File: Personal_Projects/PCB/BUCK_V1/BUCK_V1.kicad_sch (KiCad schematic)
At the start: 10 parts, among them J1 Conn_01x03_Socket, U1 AP62150WU

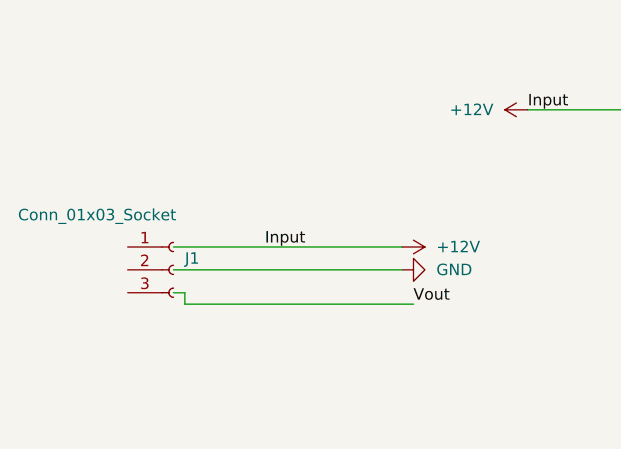
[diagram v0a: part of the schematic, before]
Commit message: lab7
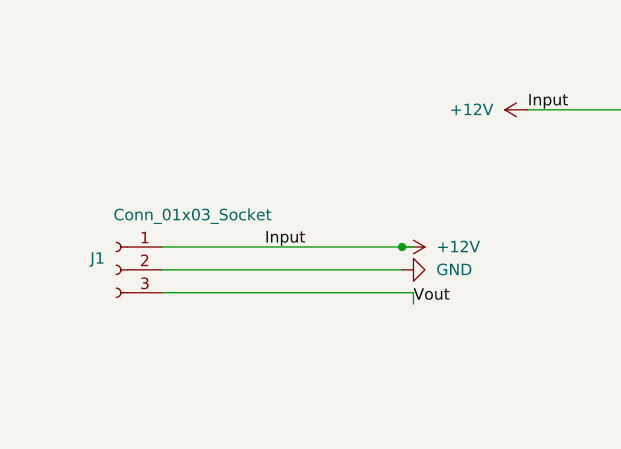
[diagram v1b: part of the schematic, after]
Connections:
- net +12V: now also J1.1 (Pin_1)
- net GND: now also J1.2 (Pin_2)
- net Vout: now also J1.3 (Pin_3)
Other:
- moved on the sheet: J1
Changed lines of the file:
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@@
+	)
+	(junction
+		(at 57.15 60.96)
+		(diameter 0)
+		(color 0 0 0 0)
 	)
 	(junction
@@
 	(wire
 		(pts
-			(xy 31.75 63.5) (xy 57.15 63.5)
+			(xy 30.48 66.04) (xy 58.42 66.04)
 		)
 		(stroke
@@
 	(wire
 		(pts
-			(xy 31.75 66.04) (xy 33.02 66.04)
-		)
-		(stroke
-			(width 0)
-			(type default)
-		)
-	)
-	(wire
-		(pts
 			(xy 146.05 41.91) (xy 166.37 41.91)
 		)
@@
 	(wire
 		(pts
-			(xy 31.75 60.96) (xy 57.15 60.96)
-		)
-		(stroke
-			(width 0)
-			(type default)
-		)
-	)
-	(wire
-		(pts
 			(xy 111.76 72.39) (xy 111.76 74.93)
 		)
@@
 	(wire
 		(pts
+			(xy 57.15 60.96) (xy 58.42 60.96)
+		)
+		(stroke
+			(width 0)
+			(type default)
+		)
+	)
+	(wire
+		(pts
 			(xy 121.92 45.72) (xy 121.92 41.91)
 		)
@@
 	(wire
 		(pts
+			(xy 30.48 60.96) (xy 57.15 60.96)
+		)
+		(stroke
+			(width 0)
+			(type default)
+		)
+	)
+	(wire
+		(pts
 			(xy 166.37 54.61) (xy 166.37 72.39)
 		)
@@
 	(wire
 		(pts
-			(xy 33.02 66.04) (xy 33.02 67.31)
-		)
-		(stroke
-			(width 0)
-			(type default)
-		)
-	)
-	(wire
-		(pts
-			(xy 33.02 67.31) (xy 58.42 67.31)
+			(xy 58.42 66.04) (xy 58.42 67.31)
 		)
 		(stroke
@@
 		(pts
 			(xy 166.37 41.91) (xy 166.37 49.53)
+		)
+		(stroke
+			(width 0)
+			(type default)
+		)
+	)
+	(wire
+		(pts
+			(xy 30.48 63.5) (xy 57.15 63.5)
 		)
 		(stroke
@@
 	(symbol
 		(lib_id "Connector:Conn_01x03_Socket")
-		(at 31.75 63.5 0)
+		(at 25.4 63.5 0)
+		(mirror y)
 		(unit 1)
 		(exclude_from_sim no)
@@
 		(dnp no)
 		(property "Reference" "J1"
-			(at 33.02 62.2299 0)
+			(at 24.13 62.2299 0)
 			(effects
 				(font
@@
 		)
 		(property "Value" "Conn_01x03_Socket"
-			(at 14.478 57.404 0)
+			(at 42.672 57.404 0)
 			(effects
 				(font
@@
 		)
 		(property "Footprint" "Connector_PinSocket_2.54mm:PinSocket_1x03_P2.54mm_Vertical"
-			(at 31.75 63.5 0)
+			(at 25.4 63.5 0)
 			(effects
 				(font
@@
 		)
 		(property "Datasheet" "~"
-			(at 31.75 63.5 0)
+			(at 25.4 63.5 0)
 			(effects
 				(font
@@
 		)
 		(property "Description" "Generic connector, single row, 01x03, script generated"
-			(at 31.75 63.5 0)
-			(effects
-				(font
+			(at 25.4 63.5 0)
+			(effects
+				(font
